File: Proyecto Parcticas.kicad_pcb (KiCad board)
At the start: 2 copper layers, 53.4 x 79.4 mm, 25 parts, among them J2 Molex_KK-254_AE-6410-06A_1x06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, J3 Baterias, U1 Sensor_de_corriente_ACS758LCB

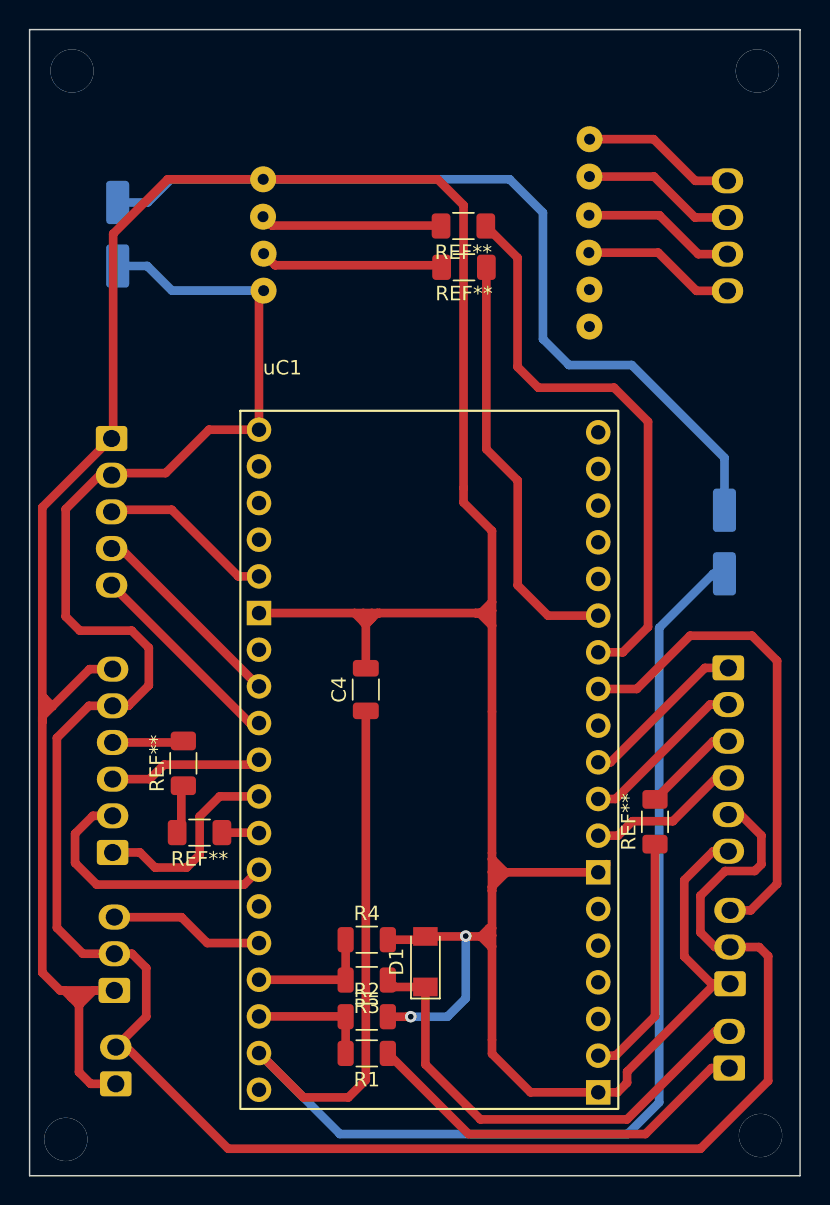
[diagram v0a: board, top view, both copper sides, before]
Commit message: Ultima super mejorada
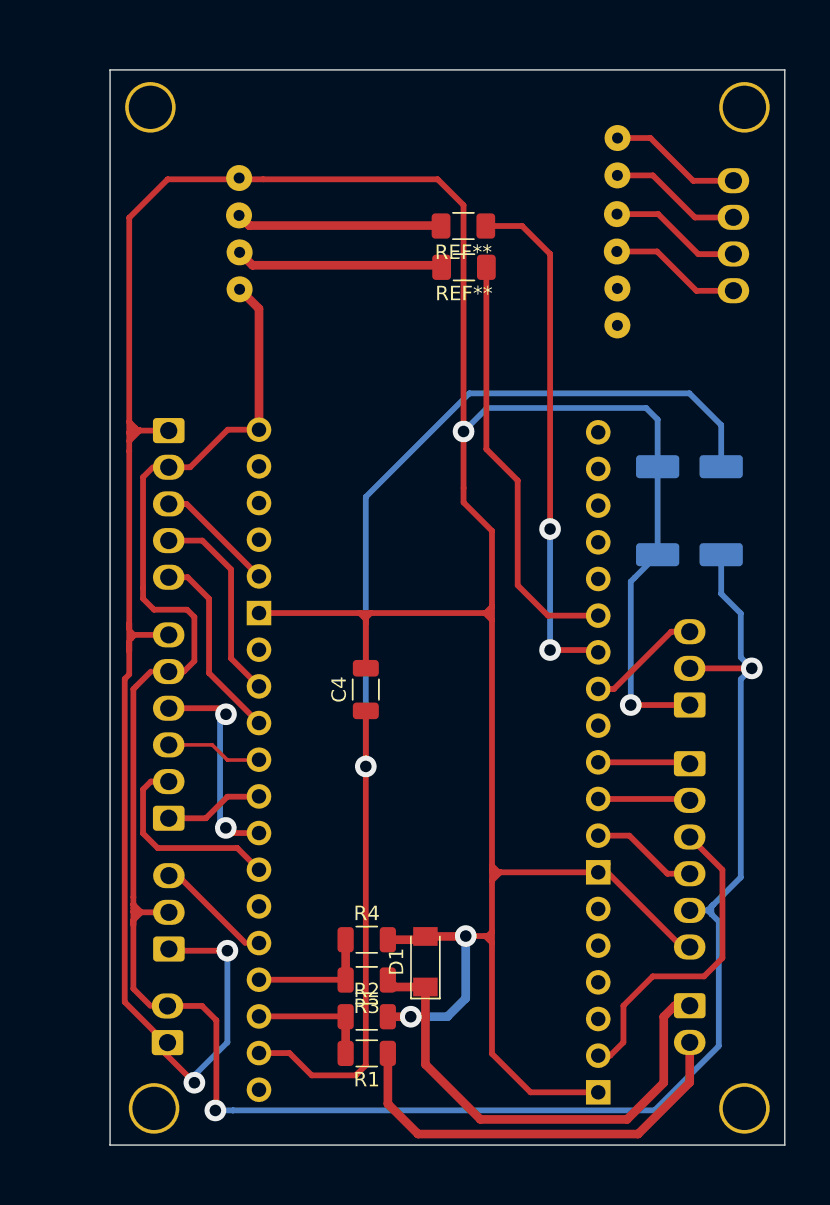
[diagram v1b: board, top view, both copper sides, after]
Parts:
- removed the REF** at (145.0, 115.3)
- removed the REF** at (177.7, 119.3)
- removed the REF** at (146.2, 120.1)
- removed uC1: Esp32s, Esp32:Esp32
- added ?: , , F.Cu at (183.9, 139.2)
- added ?: , , F.Cu at (142.7, 69.8)
- added ?: , , F.Cu at (183.9, 69.8)
- added ?: , , F.Cu at (143.0, 139.2)
- moved C2 45.4 mm to (180.1, 100.8), turned to 180 degrees
- moved S1 19.5 mm to (180.1, 106.2)
- moved J2 7.15 mm to (180.1, 115.3)
- moved C3 5.75 mm to (180.1, 94.7), turned to 180 degrees
- moved J3 5.11 mm to (180.1, 132.1), turned to -90 degrees
- moved U1 4.75 mm to (144.0, 128.2)
- moved Entrada_Alim. 4.58 mm to (143.9, 134.6)
- moved DS1 4.55 mm to (144.0, 119.1)
- moved E1 4.00 mm to (144.0, 102.4)
- moved S2 1.67 mm to (159.7, 78.5)
- moved S3 0.41 mm to (183.1, 74.9)
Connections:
- C2 pad 1: unconnected-(C2-Pad1) -> VCC
- C3 pad 1: Net-(C3-Pad1) -> EN
- D1 pad 1: BAText+ -> GND
- E1 pad 1: (no net) -> E_CLK
- E1 pad 2: (no net) -> E_DT
- E1 pad 3: (no net) -> E_SW
- E1 pad 4: (no net) -> VCC
- E1 pad 5: (no net) -> GND
- J3 pad 2: BAText+ -> BATint+
- R3 pad 1: BAText+ -> GND
- S3 pad 1: (no net) -> Net-(S2-Pad3)
- S3 pad 2: (no net) -> Net-(S2-Pad4)
- S3 pad 3: (no net) -> Net-(S2-Pad2)
- S3 pad 4: (no net) -> Net-(S2-Pad1)
- U1 pad 1: (no net) -> GND
- U1 pad 2: (no net) -> VCC
- U1 pad 3: (no net) -> S_C_OU1
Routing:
- net Net-(C3-Pad1): track 69.9 -> 0.00 mm
- net EN: track 34.7 -> 82.9 mm, vias 0 -> 1
- net BAText+: track 33.3 -> 0.00 mm
- net S_I_OUT: track 34.1 -> 7.98 mm
- net D_SDA: track 14.3 -> 7.01 mm
- net SD_SCK: track 11.7 -> 6.38 mm
- net SD_CS: track 11.7 -> 6.38 mm
- net VCC: track 163.5 -> 158.5 mm, vias 0 -> 2
- net D_DC: track 18.9 -> 14.1 mm
- net D_RES: track 11.0 -> 14.8 mm, vias 0 -> 2
- net E_SW: track 12.0 -> 8.51 mm
- net D_SCL: track 10.7 -> 7.22 mm
- net SD_MISO: track 10.7 -> 7.44 mm
- net GND: track 316.7 -> 313.5 mm, vias 2 -> 6
- net S_C_OU1: track 10.8 -> 8.19 mm
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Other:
- board size 53.4 x 79.4 mm -> 46.7 x 74.5 mm
